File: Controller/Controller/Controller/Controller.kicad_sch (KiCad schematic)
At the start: 67 parts, among them J1 Conn_02x40_Odd_Even, J2 Conn_02x20_Counter_Clockwise, J3 Conn_01x06, J4 Conn_01x05, J5 USB_A, J6 USB_C_Receptacle_USB2.0, J7 RJ45_Amphenol_RJMG1BD3B8K1ANR, U1 STM32F746IGTx, U2 LAN8720A, U3 M24C02-WMN

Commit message: changed LCDboard to Controller
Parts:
- added C23, C40: 4.7pF, Capacitor_SMD:C_0805_2012Metric_Pad1.18x1.45mm_HandSolder, symbol Device:C
- added R?: 10K, symbol Device:R
- added X?: XO32, Oscillator:Oscillator_SMD_EuroQuartz_XO32-4Pin_3.2x2.5mm, symbol Oscillator:XO32
- added Y1: 32.765Mhz, symbol Device:Crystal
- C1, C2: footprint (none) -> Capacitor_SMD:C_0805_2012Metric_Pad1.18x1.45mm_HandSolder; LCSC (none) -> C77081
- C10, C11, C12, C13, C14, C15, C16, C17, C18, C19, C20, C21, C22, C24, C25, C26, C27, C3, C4, C5, C6, C7, C8, C9: footprint (none) -> Capacitor_SMD:C_0805_2012Metric_Pad1.18x1.45mm_HandSolder
- J1: footprint (none) -> Connector_PinSocket_2.54mm:PinSocket_2x40_P2.54mm_Vertical
- J3: footprint (none) -> Connector_PinSocket_2.54mm:PinSocket_1x06_P2.54mm_Vertical
- J4: footprint (none) -> Connector_PinSocket_2.54mm:PinSocket_1x05_P2.54mm_Vertical
- J5: footprint (none) -> Connector_USB:USB_A_Molex_105057_Vertical; LCSC (none) -> C586225
- J6: footprint (none) -> Connector_USB:USB_C_Receptacle_Palconn_UTC16-G
- R1, R10, R14, R16, R18, R2, R20, R21, R23, R24, R25, R26, R3, R4, R5, R6, R7: footprint (none) -> Resistor_SMD:R_0805_2012Metric_Pad1.20x1.40mm_HandSolder
- R11: footprint (none) -> Resistor_SMD:R_0805_2012Metric_Pad1.20x1.40mm_HandSolder; LCSC (none) -> C17431
- R13, R15, R19, R22: footprint (none) -> Resistor_SMD:R_0805_2012Metric_Pad1.20x1.40mm_HandSolder; LCSC (none) -> C204544
- R27, R29: value R -> 10K; footprint (none) -> Resistor_SMD:R_0805_2012Metric_Pad1.20x1.40mm_HandSolder
- R8, R9: value 20 -> 22; footprint (none) -> Resistor_SMD:R_0805_2012Metric_Pad1.20x1.40mm_HandSolder
- gave numbers to parts that had none: 3
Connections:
- net OSC_25M is gone; now on net 25Mhz: R10.1
- net +3V3: now also R?.1, X?.4 (V+)
- net Crystal_32_in: now also C23.2, Y1.2
- net Crystal_32_out: now also C40.2, Y1.1
- net GND: now also C23.1, C40.1, X?.2 (GND)
- net Crystal_in renamed 25Mhz
- net 25Mhz: now also X?.3 (OUT)
- net Crystal_out: no longer names the net of U1.30 (PH1)
- new net: R?.2, X?.1 (EN)

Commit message: Rev 1 LCD contoller board
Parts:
- removed J1: Conn_02x40_Odd_Even, Connector_PinSocket_2.54mm:PinSocket_2x40_P2.54mm_Vertical, symbol Connector_Generic:Conn_02x40_Odd_Even
- added C41, C42: 100nF, Capacitor_SMD:C_0805_2012Metric_Pad1.18x1.45mm_HandSolder, symbol Device:C
- added J1: Conn_01x02, TerminalBlock:TerminalBlock_bornier-2_P5.08mm, symbol Connector_Generic:Conn_01x02
- J7: footprint Connector_RJ:RJ45_Amphenol_RJMG1BD3B8K1ANR -> 00_Custom_Kicad:HR913550A
- R10: value 100 -> a
- R11: value 12K1 -> 12.1Kohm
- R12, R17: value 10K -> 10Kohm; footprint (none) -> Resistor_SMD:R_0805_2012Metric_Pad1.20x1.40mm_HandSolder
- R13, R15, R19, R22: value 50 -> 50ohm
- R14, R16, R18, R20, R24: value 4K7 -> 4.7Kohm
- R21: value 1K5 -> 1.5Kohm
- R23, R25: value 330 -> 330ohm
- R26: value 47K -> 47Kohm
- R27, R29: value 10K -> 10Kohm
- R28: renamed from R?; value 10K -> 10Kohm; footprint (none) -> Resistor_SMD:R_0805_2012Metric_Pad1.20x1.40mm_HandSolder
- R8, R9: value 22 -> 22ohm
- U2: LCSC (none) -> C17146
- X1: renamed from X?; LCSC (none) -> C387396
- Y1: footprint (none) -> Crystal:Crystal_SMD_3215-2Pin_3.2x1.5mm; LCSC (none) -> C271654
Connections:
- net NRST is gone; now on net RESET: U2.15 (RST)
- net PG6 is gone; now on net Galv_Interrupt: J2.21 (Pin_21)
- net PG8 is gone; now on net Galv_Enable: J2.22 (Pin_22)
- net +3V3: now also C41.1, C42.1
- net ADDR_LED1: now also J2.11 (Pin_11)
- net ADDR_LED2: now also J2.9 (Pin_9)
- net ADDR_LED3: now also J2.7 (Pin_7); no longer J2.9 (Pin_9)
- net ADDR_LED4: now also J2.5 (Pin_5); no longer J2.11 (Pin_11), J2.7 (Pin_7)
- net ADDR_LED5: no longer J2.5 (Pin_5)
- net GND: now also C41.2, C42.2, J1.2 (Pin_2)
- net I2C1_SCL: now also J2.17 (Pin_17)
- net I2C1_SDA: now also J2.18 (Pin_18)
- net I2C2_SCL: no longer U3.6 (SCL)
- net I2C2_SDA: no longer U3.5 (SDA)
- net I2C3_SCL: now also U3.6 (SCL); no longer J2.17 (Pin_17)
- net I2C3_SDA: now also U3.5 (SDA); no longer J2.18 (Pin_18)
- net Vin: now also J1.1 (Pin_1)
- net TX-: now reaches J7.R2 (TD-), R15.2, U2.20 (TXN)
- net RX+: now reaches J7.R3 (RD+), R19.2, U2.23 (RXP)
- net TX+: now reaches J7.R1 (TD+), R13.2, U2.21 (TXP)
- net Galv_Interrupt: now reaches U1.109 (PG5)
- net Galv_Enable: now reaches U1.110 (PG6)
- net Backlight: now reaches U1.134 (PI3)
- net RX-: now reaches J7.R6 (RD-), R22.2, U2.22 (RXN)
- net PG4: no longer names the net of J2.23 (Pin_23)
- net PG5: no longer names the net of J2.24 (Pin_24)
- net RMII_RXD0 renamed RMII_RXD-
- net RMII_RXD1 renamed RMII_RXD+
- net RMII_TXD0 renamed RMII_TXD-
- net RMII_TXD1 renamed RMII_TXD+
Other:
- note removed: "Connect to some GPIO"

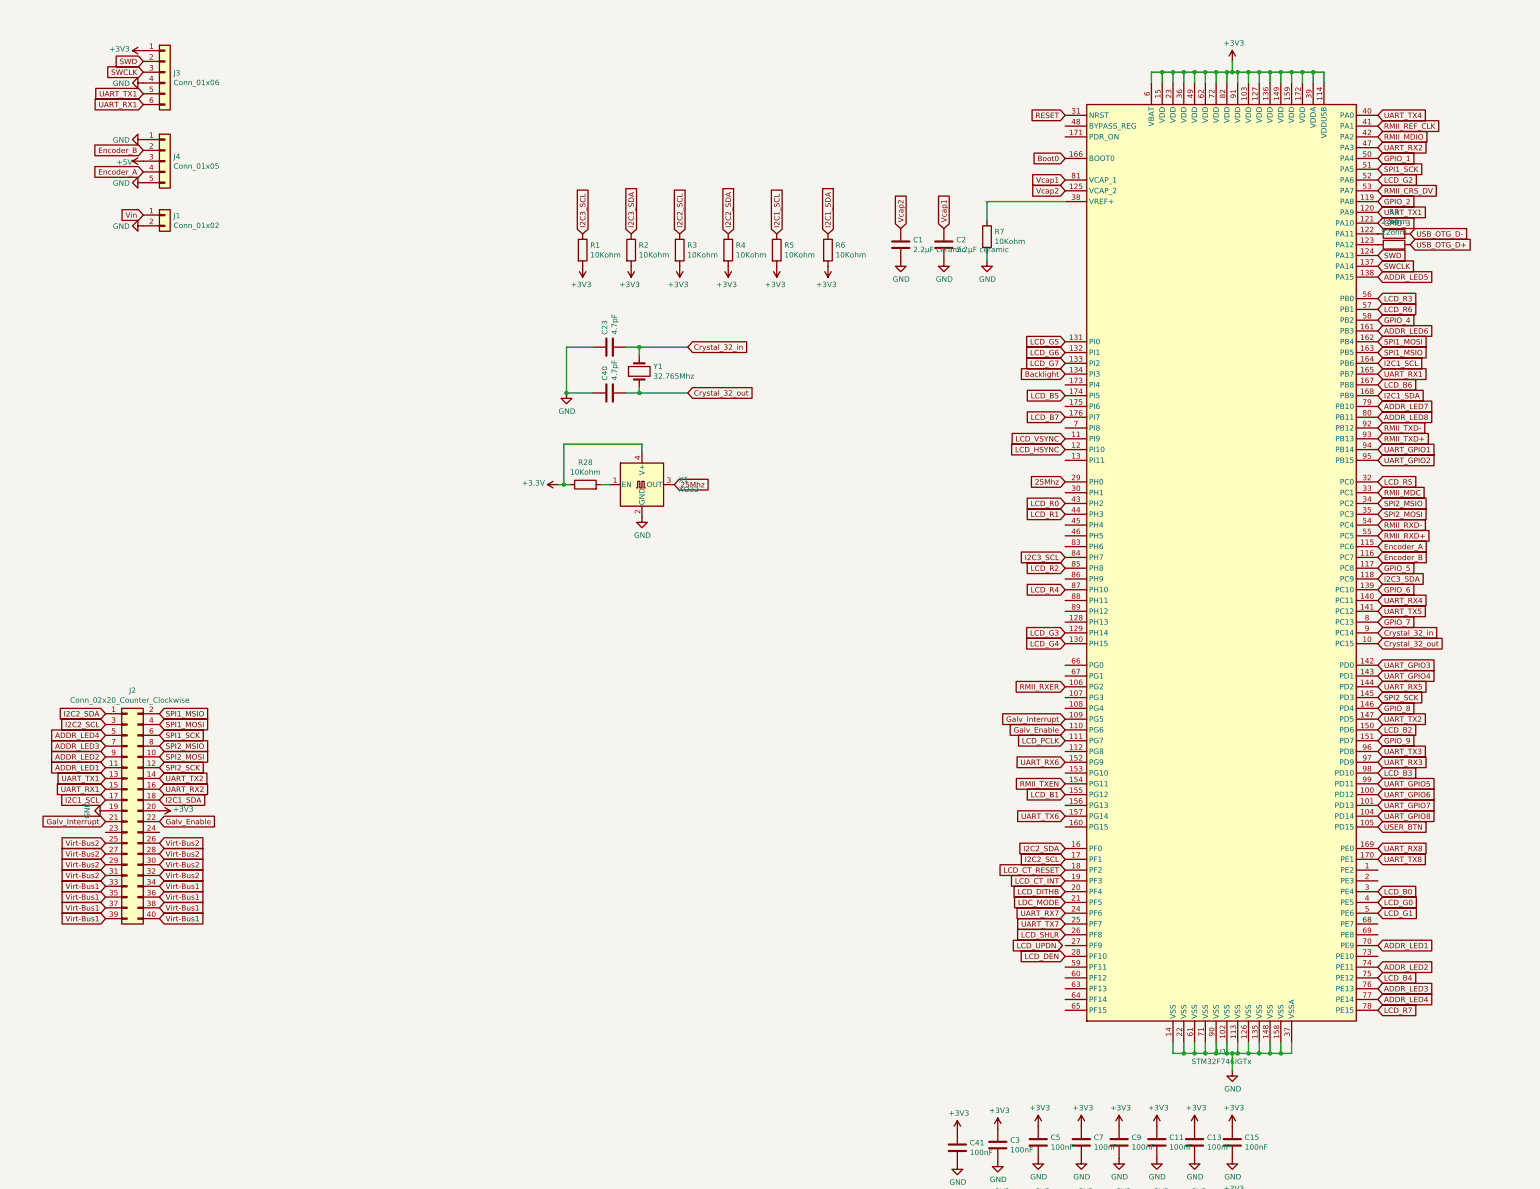
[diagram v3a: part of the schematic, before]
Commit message: ReV 2 of the contoller Board
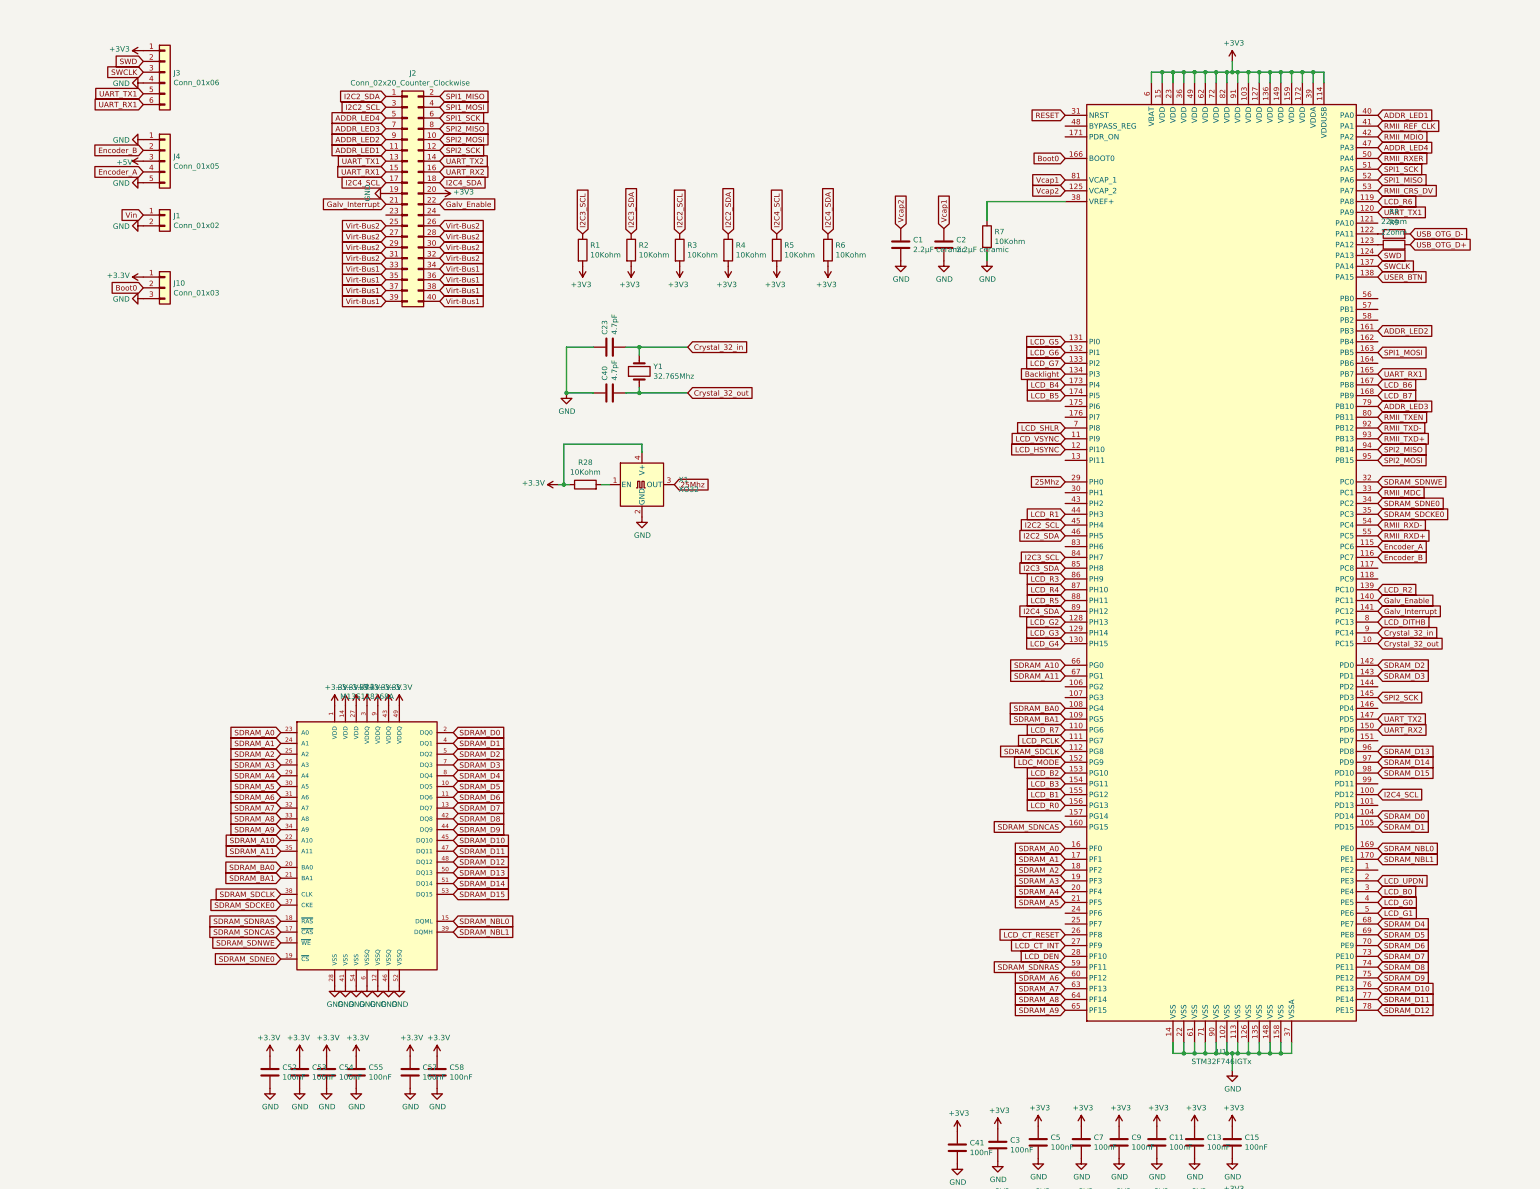
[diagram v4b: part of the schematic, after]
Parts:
- added C52, C53, C54, C55, C57, C58: 100nF, Capacitor_SMD:C_0805_2012Metric_Pad1.18x1.45mm_HandSolder, symbol Device:C
- added J10: Conn_01x03, Connector_PinSocket_2.54mm:PinSocket_1x03_P2.54mm_Vertical, symbol Connector_Generic:Conn_01x03
- added U11: M13S128168A, Package_SO:TSOP-II-54_22.2x10.16mm_P0.8mm, symbol 00_LIB:M13S128168A
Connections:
- net ADDR_LED5 is gone; now on net USER_BTN: U1.138 (PA15)
- net ADDR_LED6 is gone; now on net ADDR_LED2: U1.161 (PB3)
- net ADDR_LED7 is gone; now on net ADDR_LED3: U1.79 (PB10)
- net ADDR_LED8 is gone; now on net RMII_TXEN: U1.80 (PB11)
- net GPIO_1 is gone; now on net RMII_RXER: U1.50 (PA4)
- net GPIO_2 is gone; now on net LCD_R6: U1.119 (PA8)
- net GPIO_6 is gone; now on net LCD_R2: U1.139 (PC10)
- net GPIO_7 is gone; now on net LCD_DITHB: U1.8 (PC13)
- net UART_GPIO2 is gone; now on net SPI2_MOSI: U1.95 (PB15)
- net UART_GPIO6 is gone; now on net I2C4_SCL: U1.100 (PD12)
- net UART_RX4 is gone; now on net Galv_Enable: U1.140 (PC11)
- net UART_RX6 is gone; now on net LDC_MODE: U1.152 (PG9)
- net UART_TX4 is gone; now on net ADDR_LED1: U1.40 (PA0)
- net UART_TX5 is gone; now on net Galv_Interrupt: U1.141 (PC12)
- net +3V3: now also C52.1, C53.1, C54.1, C55.1, C57.1, C58.1, J10.1 (Pin_1), U11.1 (VDD), U11.14 (VDD), U11.27 (VDD), U11.3 (VDDQ), U11.43 (VDDQ), U11.49 (VDDQ), U11.9 (VDDQ)
- net ADDR_LED1: no longer U1.70 (PE9)
- net ADDR_LED2: no longer U1.74 (PE11)
- net ADDR_LED3: no longer U1.76 (PE13)
- net ADDR_LED4: now also U1.47 (PA3); no longer U1.77 (PE14)
- net Boot0: now also J10.2 (Pin_2)
- net GND: now also C52.2, C53.2, C54.2, C55.2, C57.2, C58.2, J10.3 (Pin_3), U11.12 (VSSQ), U11.28 (VSS), U11.41 (VSS), U11.46 (VSSQ), U11.52 (VSSQ), U11.54 (VSS), U11.6 (VSSQ)
- net Galv_Enable: no longer U1.110 (PG6)
- net Galv_Interrupt: no longer U1.109 (PG5)
- net I2C2_SCL: now also U1.45 (PH4); no longer U1.17 (PF1)
- net I2C2_SDA: now also U1.46 (PH5); no longer U1.16 (PF0)
- net I2C3_SDA: now also U1.85 (PH8); no longer U1.118 (PC9)
- net LCD_B2: now also U1.153 (PG10); no longer U1.150 (PD6)
- net LCD_B3: now also U1.154 (PG11); no longer U1.98 (PD10)
- net LCD_B4: now also U1.173 (PI4); no longer U1.75 (PE12)
- net LCD_B7: now also U1.168 (PB9); no longer U1.176 (PI7)
- net LCD_CT_INT: now also U1.27 (PF9); no longer U1.19 (PF3)
- net LCD_CT_RESET: now also U1.26 (PF8); no longer U1.18 (PF2)
- net LCD_DITHB: no longer U1.20 (PF4)
- net LCD_G2: now also U1.128 (PH13); no longer U1.52 (PA6)
- net LCD_R0: now also U1.156 (PG13); no longer U1.43 (PH2)
- net LCD_R2: no longer U1.85 (PH8)
- net LCD_R3: now also U1.86 (PH9); no longer U1.56 (PB0)
- net LCD_R5: now also U1.88 (PH11); no longer U1.32 (PC0)
- net LCD_R6: no longer U1.57 (PB1)
- net LCD_R7: now also U1.110 (PG6); no longer U1.78 (PE15)
- net LCD_SHLR: now also U1.7 (PI8); no longer U1.26 (PF8)
- net LCD_UPDN: now also U1.2 (PE3)
- net LDC_MODE: no longer U1.21 (PF5)
- net RMII_RXER: no longer U1.106 (PG2)
- net RMII_TXEN: no longer U1.154 (PG11)
- net SPI1_MOSI: now also U1.163 (PB5); no longer U1.162 (PB4)
- net SPI2_MOSI: no longer U1.35 (PC3)
- net UART_RX2: now also U1.150 (PD6); no longer U1.47 (PA3)
- net USER_BTN: no longer U1.105 (PD15)
- net SDRAM_BA0: now reaches U1.108 (PG4)
- net SDRAM_BA0: now also U11.20 (BA0)
- net SDRAM_SDCLK: now reaches U1.112 (PG8)
- net SDRAM_SDCLK: now also U11.38 (CLK)
- net SDRAM_SDNCAS: now reaches U1.160 (PG15)
- net SDRAM_SDNCAS: now also U11.17 (~CAS~)
- net SDRAM_SDNRAS: now reaches U1.59 (PF11)
- net SDRAM_SDNRAS: now also U11.18 (~RAS~)
- net SDRAM_A6: now reaches U1.60 (PF12)
- net SDRAM_A6: now also U11.31 (A6)
- net SDRAM_A7: now reaches U1.63 (PF13)
- net SDRAM_A7: now also U11.32 (A7)
- net SDRAM_A8: now reaches U1.64 (PF14)
- net SDRAM_A8: now also U11.33 (A8)
- net SDRAM_A9: now reaches U1.65 (PF15)
- net SDRAM_A9: now also U11.34 (A9)
- net SDRAM_A10: now reaches U1.66 (PG0)
- net SDRAM_A10: now also U11.22 (A10)
- net SDRAM_A11: now reaches U1.67 (PG1)
- net SDRAM_A11: now also U11.35 (A11)
- net SDRAM_D4: now reaches U1.68 (PE7)
- net SDRAM_D4: now also U11.8 (DQ4)
- net SDRAM_D5: now reaches U1.69 (PE8)
- net SDRAM_D5: now also U11.10 (DQ5)
- net SDRAM_D7: now reaches U1.73 (PE10)
- net SDRAM_D7: now also U11.13 (DQ7)
- net I2C4_SDA: now reaches U1.89 (PH12)
- net I2C4_SDA: now also J2.18 (Pin_18), R6.1
- net GPIO_3: no longer names the net of U1.121 (PA10)
- net GPIO_4: no longer names the net of U1.58 (PB2)
- net GPIO_5: no longer names the net of U1.117 (PC8)
- net GPIO_8: no longer names the net of U1.146 (PD4)
- net GPIO_9: no longer names the net of U1.151 (PD7)
- net I2C1_SCL renamed I2C4_SCL
- net I2C4_SCL: no longer U1.164 (PB6)
- removed net I2C1_SDA: J2.18 (Pin_18), R6.1, U1.168 (PB9)
- net SPI1_MSIO renamed SPI1_MISO
- net SPI1_MISO: now also U1.52 (PA6); no longer U1.163 (PB5)
- net SPI2_MSIO renamed SDRAM_SDNE0
- net SDRAM_SDNE0: now also U11.19 (~CS~); no longer J2.8 (Pin_8)
- net UART_GPIO1 renamed SPI2_MISO
- net SPI2_MISO: now also J2.8 (Pin_8)
- net UART_GPIO3 renamed SDRAM_D2
- net SDRAM_D2: now also U11.5 (DQ2)
- net UART_GPIO4 renamed SDRAM_D3
- net SDRAM_D3: now also U11.7 (DQ3)
- net UART_GPIO5: no longer names the net of U1.99 (PD11)
- net UART_GPIO7: no longer names the net of U1.101 (PD13)
- net UART_GPIO8 renamed SDRAM_D0
- net SDRAM_D0: now also U11.2 (DQ0)
- net UART_RX3 renamed SDRAM_D14
- net SDRAM_D14: now also U11.51 (DQ14)
- net UART_RX5: no longer names the net of U1.144 (PD2)
- net UART_RX7: no longer names the net of U1.24 (PF6)
- net UART_RX8 renamed SDRAM_NBL0
- net SDRAM_NBL0: now also U11.15 (DQML)
- net UART_TX3 renamed SDRAM_D13
- net SDRAM_D13: now also U11.50 (DQ13)
- net UART_TX6: no longer names the net of U1.157 (PG14)
- net UART_TX7: no longer names the net of U1.25 (PF7)
- net UART_TX8 renamed SDRAM_NBL1
- net SDRAM_NBL1: now also U11.39 (DQMH)
- new net SDRAM_A0: U1.16 (PF0), U11.23 (A0)
- new net SDRAM_A1: U1.17 (PF1), U11.24 (A1)
- new net SDRAM_A2: U1.18 (PF2), U11.25 (A2)
- new net SDRAM_A3: U1.19 (PF3), U11.26 (A3)
- new net SDRAM_A4: U1.20 (PF4), U11.29 (A4)
- new net SDRAM_A5: U1.21 (PF5), U11.30 (A5)
- new net SDRAM_BA1: U1.109 (PG5), U11.21 (BA1)
- new net SDRAM_D1: U1.105 (PD15), U11.4 (DQ1)
- new net SDRAM_D10: U1.76 (PE13), U11.45 (DQ10)
- new net SDRAM_D11: U1.77 (PE14), U11.47 (DQ11)
- new net SDRAM_D12: U1.78 (PE15), U11.48 (DQ12)
- new net SDRAM_D15: U1.98 (PD10), U11.53 (DQ15)
- new net SDRAM_D6: U1.70 (PE9), U11.11 (DQ6)
- new net SDRAM_D8: U1.74 (PE11), U11.42 (DQ8)
- new net SDRAM_D9: U1.75 (PE12), U11.44 (DQ9)
- new net SDRAM_SDCKE0: U1.35 (PC3), U11.37 (CKE)
- new net SDRAM_SDNWE: U1.32 (PC0), U11.16 (~WE~)
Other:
- moved on the sheet: J2

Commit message: Rev 3 Pcb's
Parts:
- added R46: 130Kohm, Resistor_SMD:R_0805_2012Metric_Pad1.20x1.40mm_HandSolder, symbol Device:R
- added R47: 15Kohm, Resistor_SMD:R_0805_2012Metric_Pad1.20x1.40mm_HandSolder, symbol Device:R
- C1, C2: Orderd (none) -> 10
- C10, C11, C12, C13, C14, C15, C16, C17, C18, C19, C20, C21, C22, C24, C25, C26, C27, C3, C4, C41, C42, C43, C5, C52, C53, C54, C55, C57, C58, C6, C7, C8, C9: Orderd (none) -> 1000
- C23, C40, R13, R15, R19, R22: Orderd (none) -> 50
- J5, Y1: Orderd (none) -> 4
- J6: Orderd (none) -> 20
- J7: LCSC (none) -> C163507; Orderd (none) -> 5
- R10: value a -> 100ohm
- R11: LCSC C17431 -> C103953; Orderd (none) -> 100
- R8, R9: Orderd (none) -> 100
- U11: value M13S128168A -> IS42S16400J
- U2: Orderd (none) -> 4 mouser/farnell
- X1: value XO32 -> XO25; Orderd (none) -> 4
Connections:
- net GND: now also R47.2
- net Vin: now also R46.1
- net Vinsense: now reaches U1.43 (PH2)
- net Vinsense: now also R46.2, R47.1
- net Power3: now reaches U1.56 (PB0)
- net Power2: now reaches U1.57 (PB1)

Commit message: Final Version Tested
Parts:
- removed C17, C18, C19, C20, C21, C22, C24, C25, C52, C53, C54, C55, C57, C58: 100nF, Capacitor_SMD:C_0805_2012Metric_Pad1.18x1.45mm_HandSolder, symbol Device:C
- removed J1: Conn_01x02, TerminalBlock:TerminalBlock_bornier-2_P5.08mm, symbol Connector_Generic:Conn_01x02
- removed J10: Conn_01x03, Connector_PinSocket_2.54mm:PinSocket_1x03_P2.54mm_Vertical, symbol Connector_Generic:Conn_01x03
- removed J2: Conn_02x20_Counter_Clockwise, Connector_PinSocket_2.54mm:PinSocket_2x20_P2.54mm_Vertical, symbol Connector_Generic:Conn_02x20_Odd_Even
- removed J3: Conn_01x06, Connector_PinSocket_2.54mm:PinSocket_1x06_P2.54mm_Vertical, symbol Connector_Generic:Conn_01x06
- removed J4: Conn_01x05, Connector_PinSocket_2.54mm:PinSocket_1x05_P2.54mm_Vertical, symbol Connector_Generic:Conn_01x05
- removed J5: USB_A, Connector_USB:USB_A_Molex_105057_Vertical, symbol Connector:USB_A
- removed J6: USB_C_Receptacle_USB2.0, Connector_USB:USB_C_Receptacle_Palconn_UTC16-G, symbol Connector:USB_C_Receptacle_USB2.0
- removed J7: RJ45_Amphenol_RJMG1BD3B8K1ANR, 00_Custom_Kicad:HR913550A, symbol Connector:RJ45_Amphenol_RJMG1BD3B8K1ANR
- removed R10: 100ohm, Resistor_SMD:R_0805_2012Metric_Pad1.20x1.40mm_HandSolder, symbol Device:R
- removed R11: 12.1Kohm, Resistor_SMD:R_0805_2012Metric_Pad1.20x1.40mm_HandSolder, symbol Device:R
- removed R12, R17: 10Kohm, Resistor_SMD:R_0805_2012Metric_Pad1.20x1.40mm_HandSolder, symbol Device:R
- removed R13, R15, R19, R22: 50ohm, Resistor_SMD:R_0805_2012Metric_Pad1.20x1.40mm_HandSolder, symbol Device:R
- removed R14, R16, R18, R20, R24: 4.7Kohm, Resistor_SMD:R_0805_2012Metric_Pad1.20x1.40mm_HandSolder, symbol Device:R
- removed R21: 1.5Kohm, Resistor_SMD:R_0805_2012Metric_Pad1.20x1.40mm_HandSolder, symbol Device:R
- removed R23, R25: 330ohm, Resistor_SMD:R_0805_2012Metric_Pad1.20x1.40mm_HandSolder, symbol Device:R
- removed R26: 47Kohm, Resistor_SMD:R_0805_2012Metric_Pad1.20x1.40mm_HandSolder, symbol Device:R
- removed R46: 130Kohm, Resistor_SMD:R_0805_2012Metric_Pad1.20x1.40mm_HandSolder, symbol Device:R
- removed R47: 15Kohm, Resistor_SMD:R_0805_2012Metric_Pad1.20x1.40mm_HandSolder, symbol Device:R
- removed U11: IS42S16400J, Package_SO:TSOP-II-54_22.2x10.16mm_P0.8mm, symbol 00_LIB:M13S128168A
- removed U2: LAN8720A, Package_DFN_QFN:QFN-24-1EP_4x4mm_P0.5mm_EP2.6x2.6mm, symbol Interface_Ethernet:LAN8720A
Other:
- sheet LCD renamed LCD Connectors
- added sheet CONNECTIONS (CONNECTIONS.kicad_sch)
- added sheet NETWORK (NETWORK.kicad_sch)
- added sheet Power (Power.kicad_sch)
- added sheet SDRAM (SDRAM.kicad_sch)
- sheet LCD Connectors: file LCD.kicad_sch -> LCDConnectors.kicad_sch
- note added: "Clock Generation"
- note added: "Decoupling"
- note added: "I2C Pullups"
- note added: "MCU"
- note removed: "LAN PORT"
- note removed: "USB"
- moved on the sheet: C1, C10, C11, C12, C13, C14, C15, C16, C2, C23, C26, C27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
